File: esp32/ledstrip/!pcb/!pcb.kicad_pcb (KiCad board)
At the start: 2 copper layers, 100 x 100 mm, 16 parts, among them J1 Barrel_Jack_Switch, J2 Conn_01x03, SW1 SW_SPST, U1 ESP32 MINI, U2 INMP441

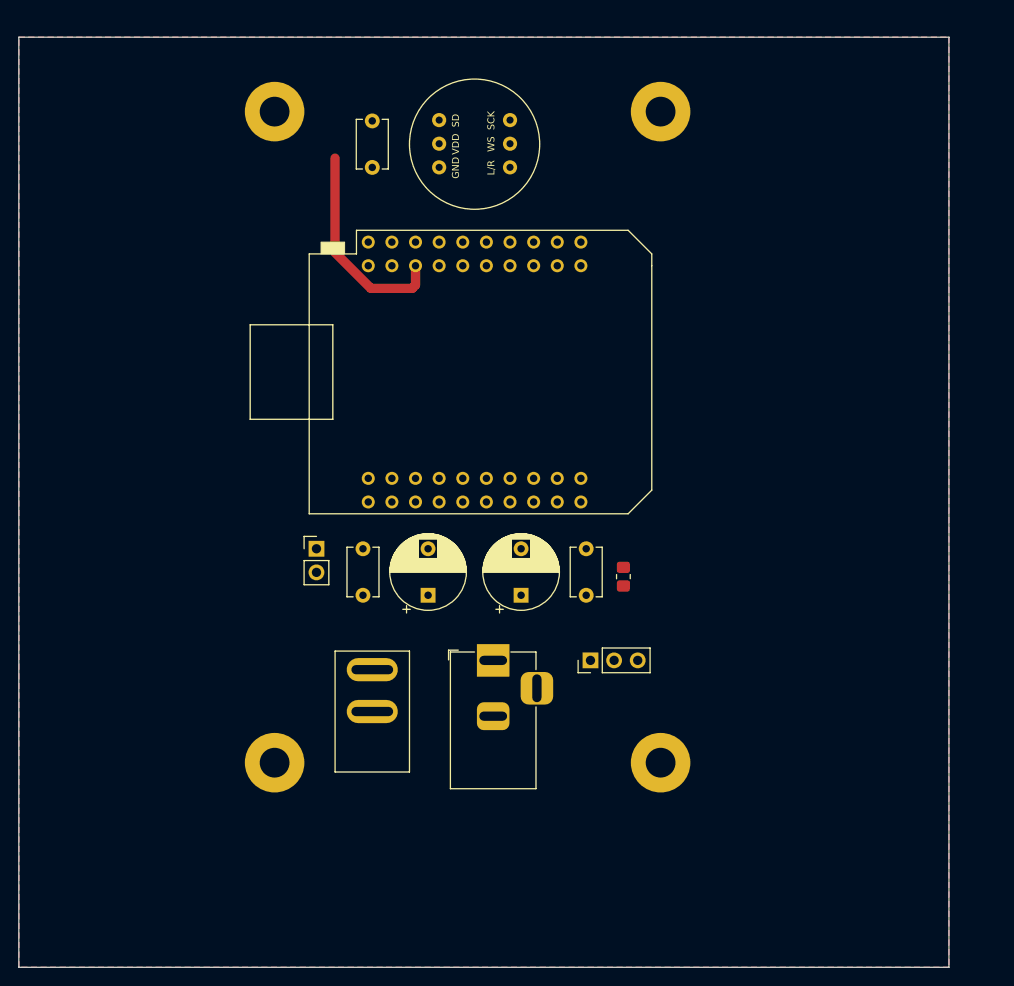
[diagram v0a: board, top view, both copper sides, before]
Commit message: ledstrip: Start routing
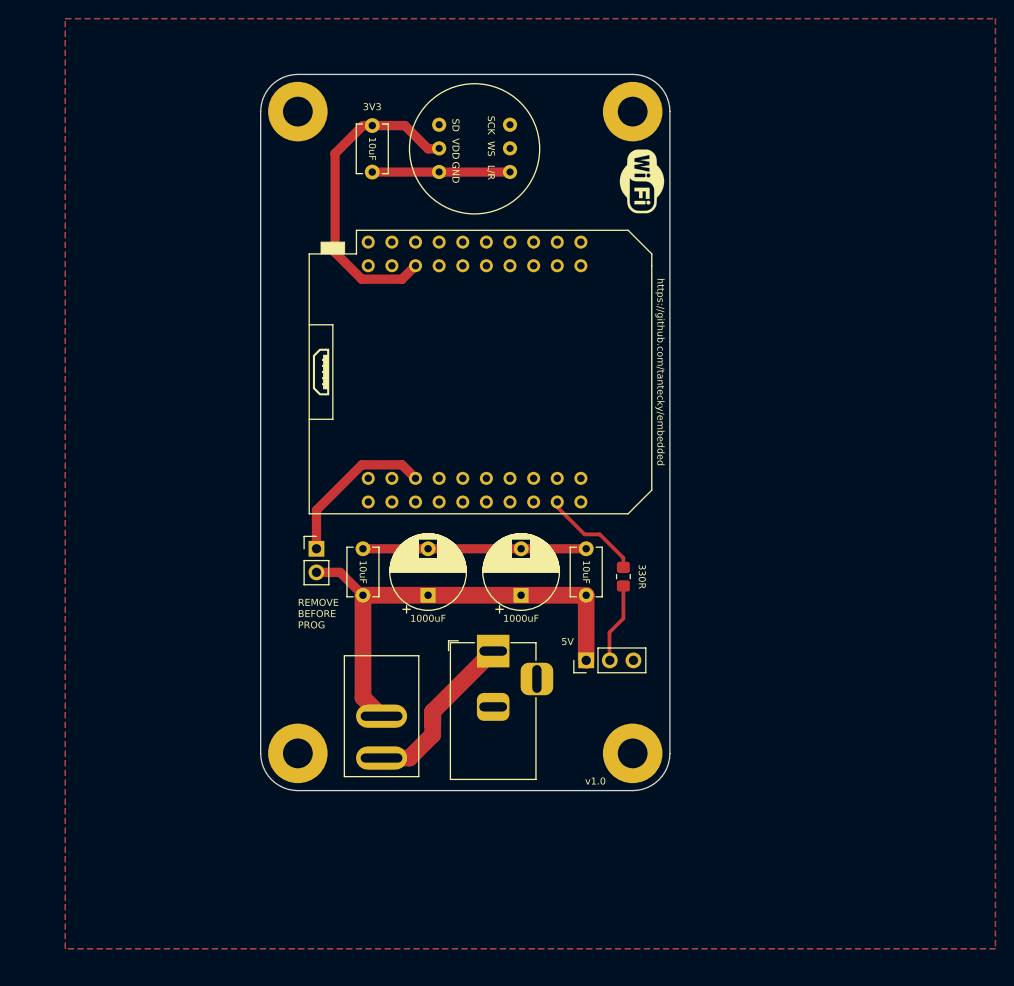
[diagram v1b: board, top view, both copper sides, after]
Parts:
- added G***: LOGO, _my:microusb, F.Cu at (52.5, 81.0)
- added G***: LOGO, _my:wifi, F.Cu at (87.0, 60.5)
- moved H3 3.16 mm to (86.0, 122.0)
- moved H1 3.00 mm to (86.0, 53.0)
- moved H4 2.69 mm to (50.0, 122.0)
- moved H2 2.50 mm to (50.0, 53.0)
- moved SW1 1.12 mm to (59.0, 118.0), turned to 270 degrees
- moved J1 1.00 mm to (71.0, 111.0)
- moved C5 0.50 mm to (58.0, 54.5)
- moved U2 0.50 mm to (69.0, 57.0)
- moved J2 0.46 mm to (81.0, 112.0)
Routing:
- net +5V: track 0.00 -> 50.8 mm
- net GND: track 0.00 -> 38.8 mm
- net Net-(J1-Pad1): track 0.00 -> 21.7 mm
- net Net-(JP1-Pad1): track 0.00 -> 17.4 mm
- net +3V3: track 22.6 -> 34.6 mm
- net STRIP: track 0.00 -> 10.9 mm
- net Net-(J2-Pad2): track 0.00 -> 8.64 mm
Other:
- board size 100 x 100 mm -> 44 x 77 mm
- board text added: "1000uF"
- board text added: "10uF"
- board text added: "330R"
- board text added: "3V3"
- board text added: "5V"
- board text added: "REMOVE BEFORE PROG"
- board text added: "https://github.com/tantecky/embedded"
- board text added: "v1.0"
